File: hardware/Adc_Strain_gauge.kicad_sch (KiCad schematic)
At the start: 16 parts, among them J12 Load Cell 2, J4 Load Cell 3, J6 Load Cell 1, U3 ADS131M03IRUKx

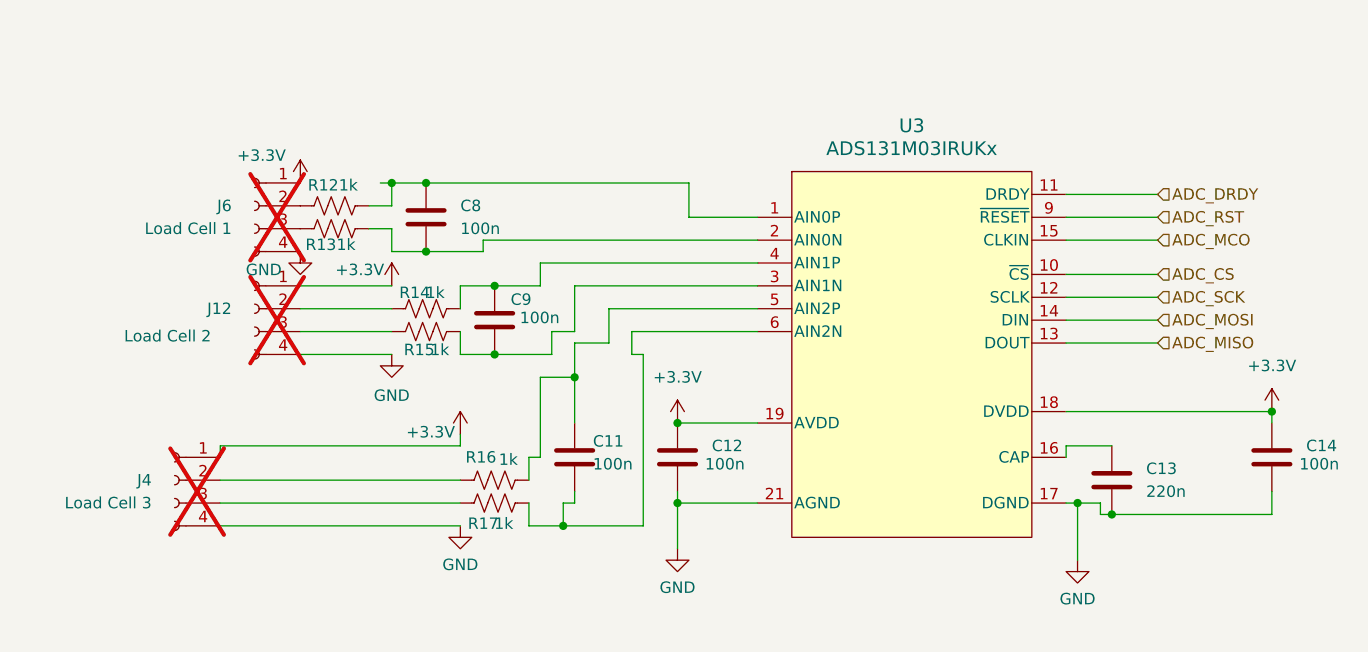
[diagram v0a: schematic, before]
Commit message: Stylistic changes
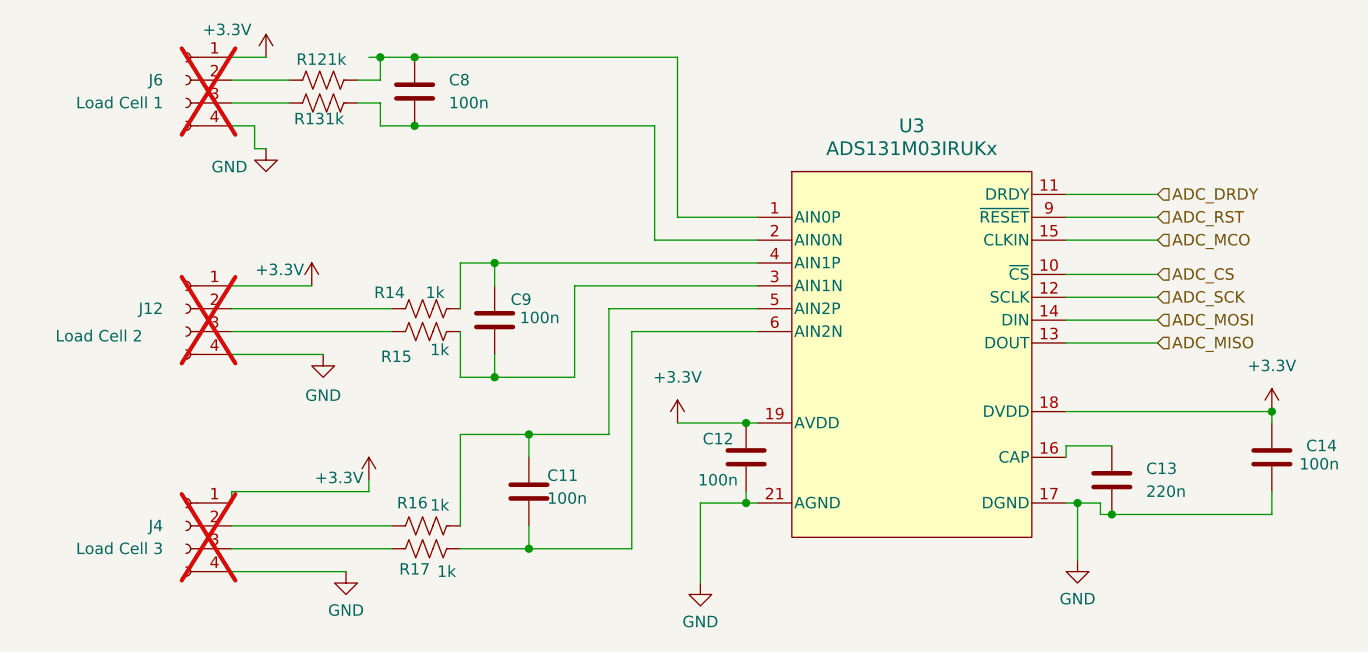
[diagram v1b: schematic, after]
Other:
- moved on the sheet: C11, C12, C8, J12, J4, J6, R12, R13, R16, R17
